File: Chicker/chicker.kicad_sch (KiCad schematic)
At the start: 0 parts

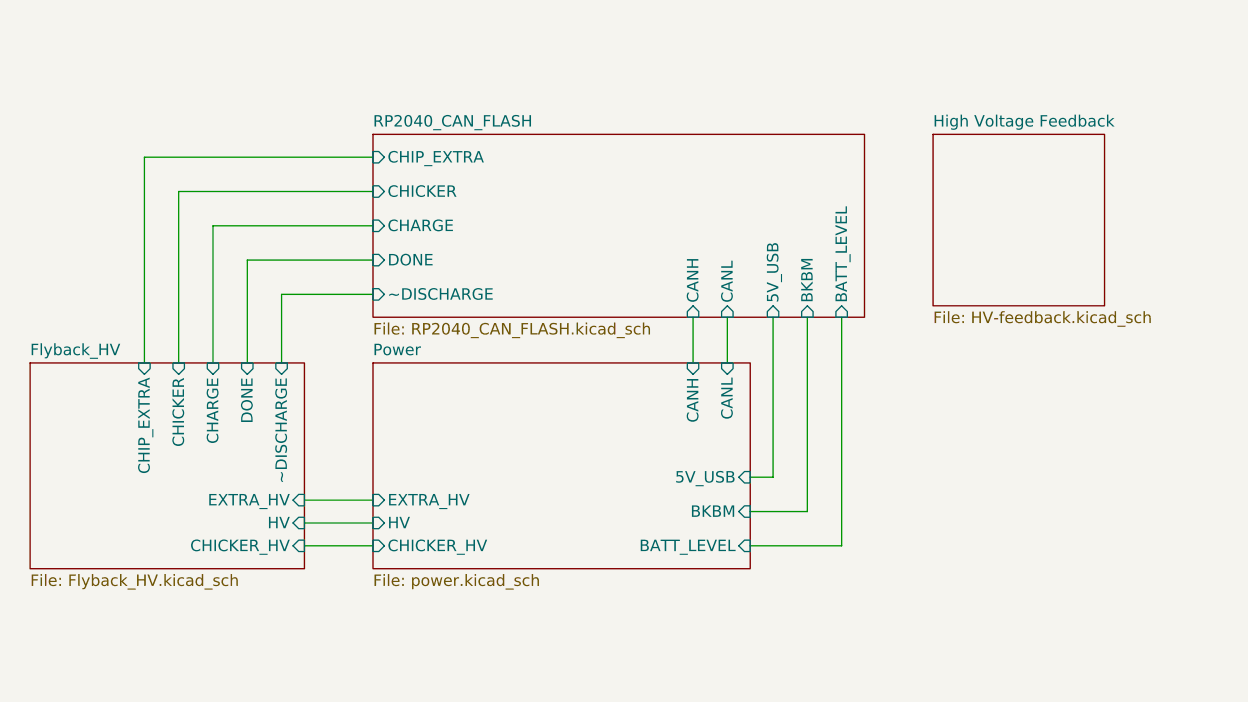
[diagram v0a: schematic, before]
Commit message: chicker v1.1 updates
nearly done, need to fix rules
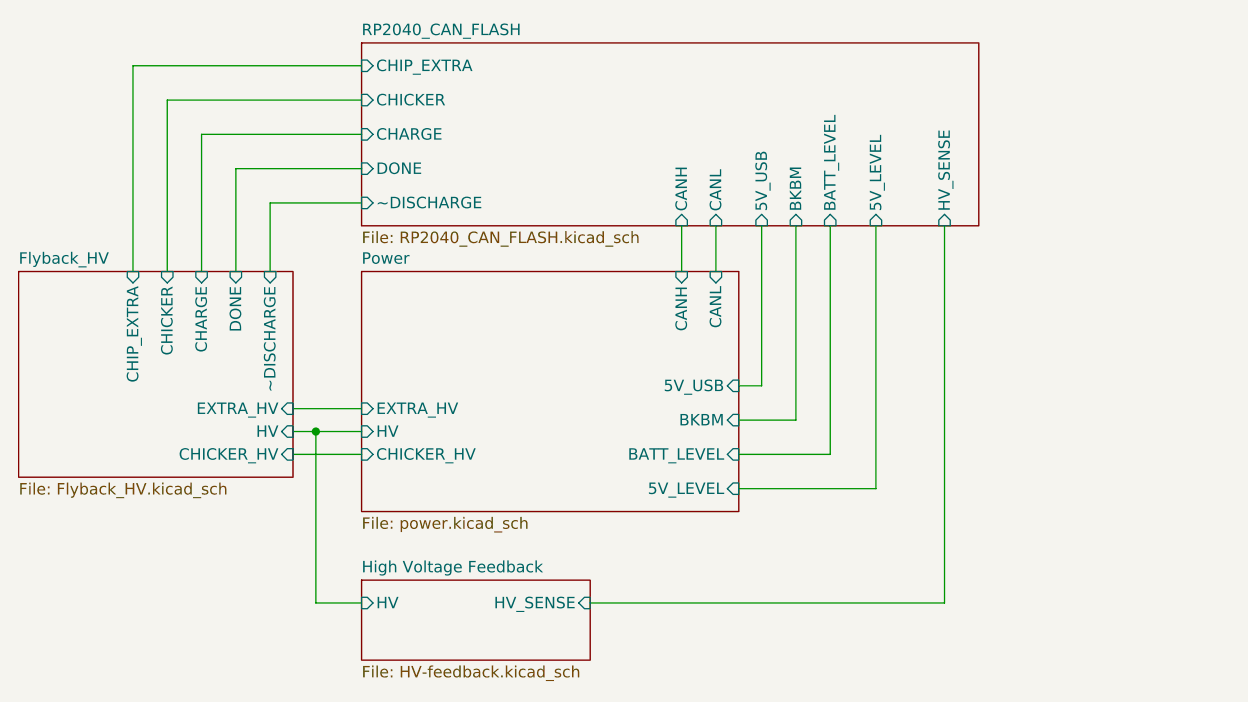
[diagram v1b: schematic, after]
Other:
- sheet High Voltage Feedback ports: added HV, HV_SENSE; removed none
- sheet Power ports: added 5V_LEVEL; removed none
- sheet RP2040_CAN_FLASH ports: added 5V_LEVEL, HV_SENSE; removed none
